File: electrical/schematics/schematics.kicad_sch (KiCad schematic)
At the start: 18 parts, among them SW101 , SW102 CHAVE MOTOR, SW103 

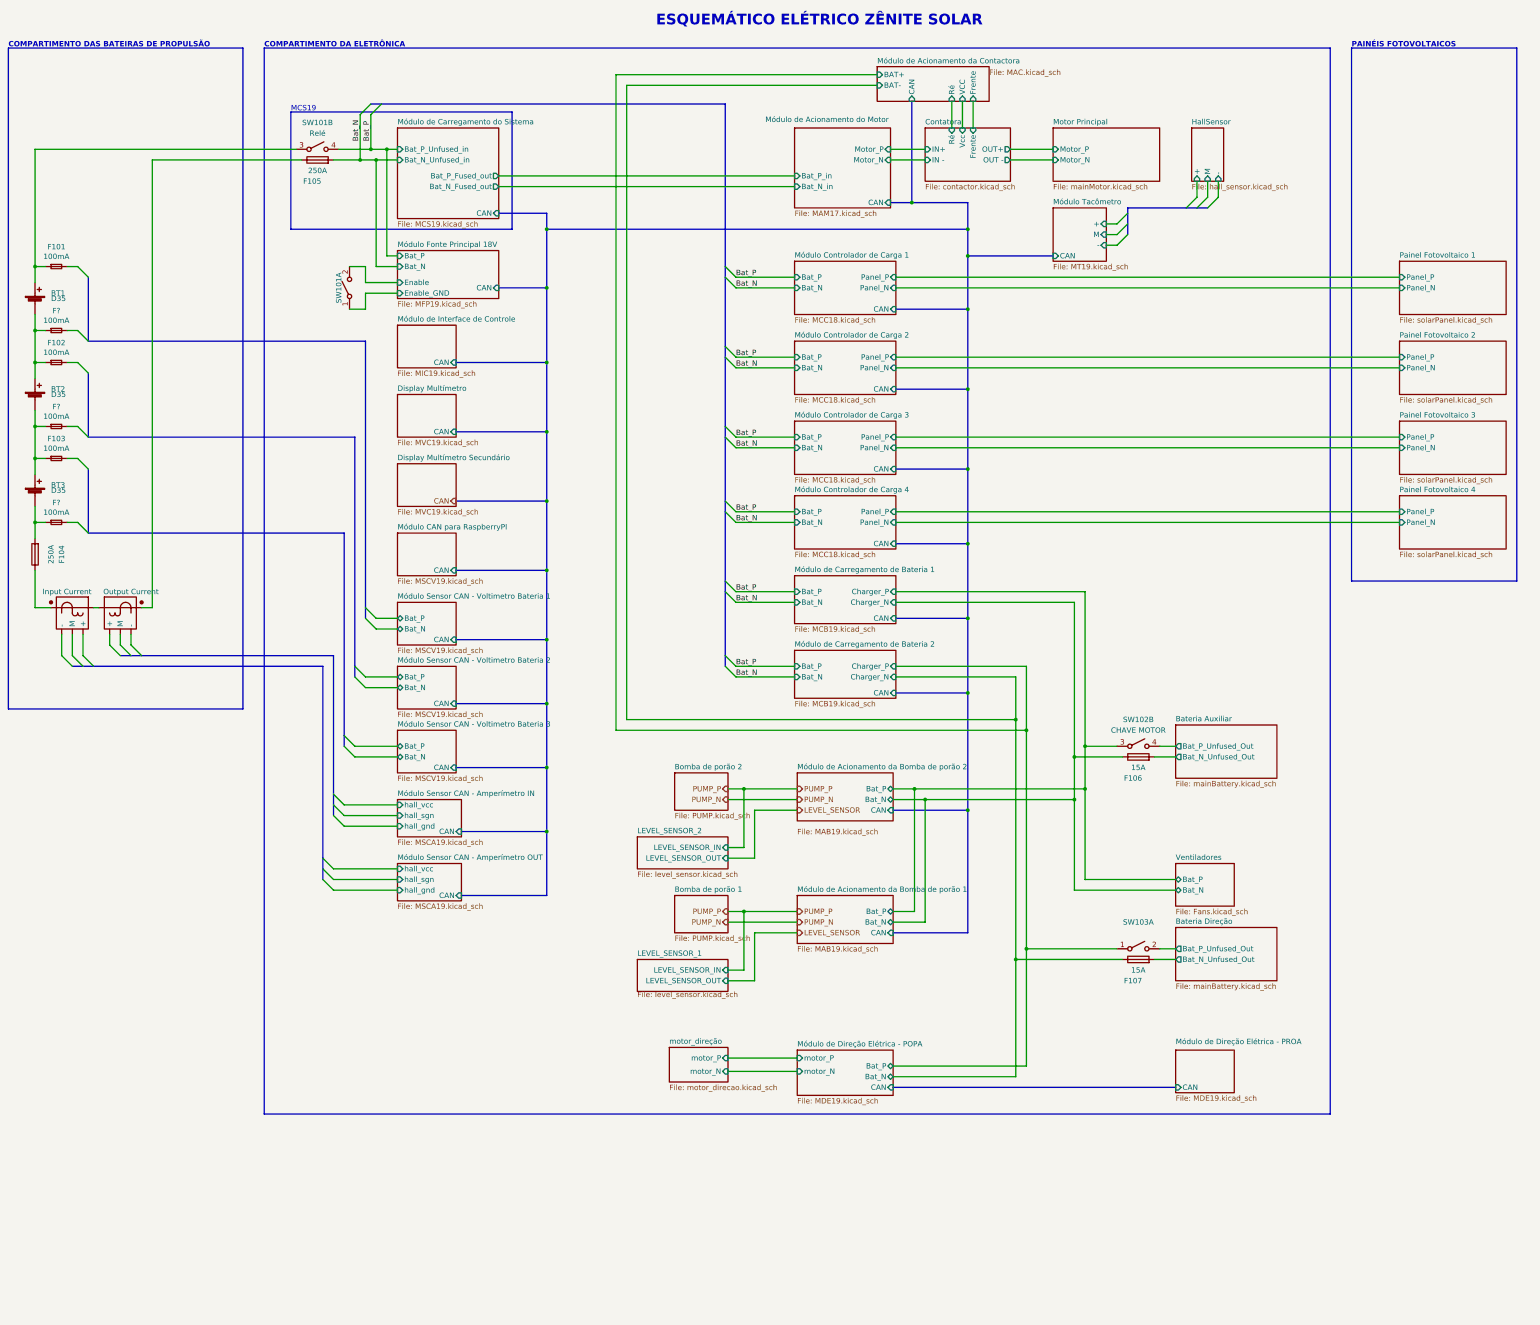
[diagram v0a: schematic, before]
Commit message: DSB 2022 ITA
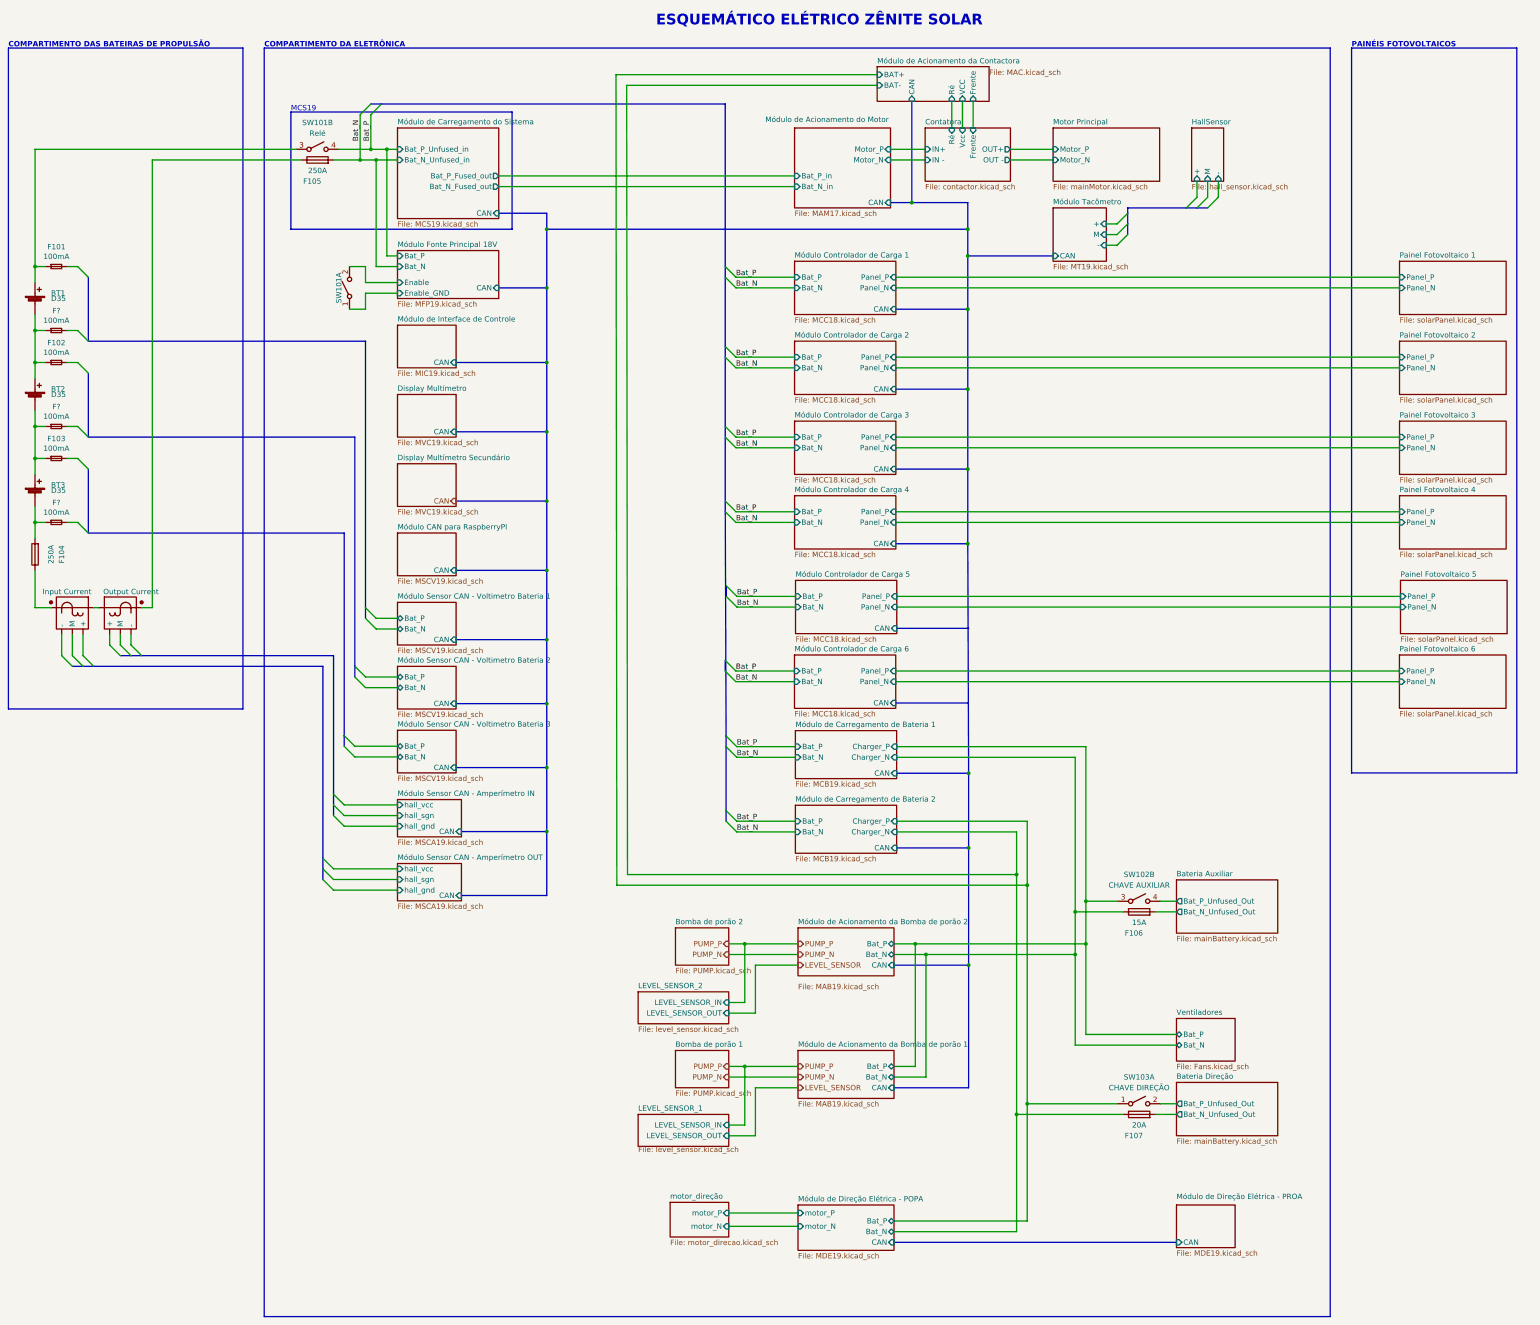
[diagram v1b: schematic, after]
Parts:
- F107: value 15A -> 20A
- SW102: value CHAVE MOTOR -> CHAVE AUXILIAR
- SW103: value (none) -> CHAVE DIREÇÃO
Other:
- added sheet Módulo Controlador de Carga 5 (MCC18.kicad_sch)
- added sheet Módulo Controlador de Carga 6 (MCC18.kicad_sch)
- added sheet Painel Fotovoltaico 5 (solarPanel.kicad_sch)
- added sheet Painel Fotovoltaico 6 (solarPanel.kicad_sch)
- moved on the sheet: F106, F107, SW102B, SW103A
